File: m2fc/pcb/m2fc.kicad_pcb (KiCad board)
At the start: 4 copper layers, 100 x 70 mm, 347 parts, among them IC101 ADP3335, IC102 STM32F405VGT, IC103 ADP3335, IC201 AD8226, IC202 AD8656, IC203 AD8541, IC204 AD8226, IC205 AD8656, IC206 AD8541, IC207 AD8226, IC208 AD8656, IC209 AD8541, IC301 ADXL375, IC302 ADXL345, IC303 MS5611-01BA03, IC304 HMC5883L, IC305 L3G4200D, IC401 ADuM5201, IC402 ADuM1201, IC601 AD8495, IC602 AD8656, IC603 AD8495, IC604 AD8656, IC605 AD8495, IC606 AD8656, P101 CONN_2, P102 CONN_2, P103 CONN_2, P104 SWD, P201 CONN_4, P202 CONN_4, P203 CONN_4, P401 CONN_4, P402 CONN_2, P403 CONN_4, P501 CONN_2, P502 CONN_2, P503 CONN_2, P601 CONN_2, P602 CONN_2, P603 CONN_2, Q501 MOSFET_P, Q502 MOSFET_N, Q503 MOSFET_P, Q504 MOSFET_N, Q505 MOSFET_P, Q506 MOSFET_N, U106 MICROSD, U107 MOUNT, U108 MOUNT, U109 MOUNT, U110 MOUNT, U111 MOUNT, U112 MOUNT, X101 8M

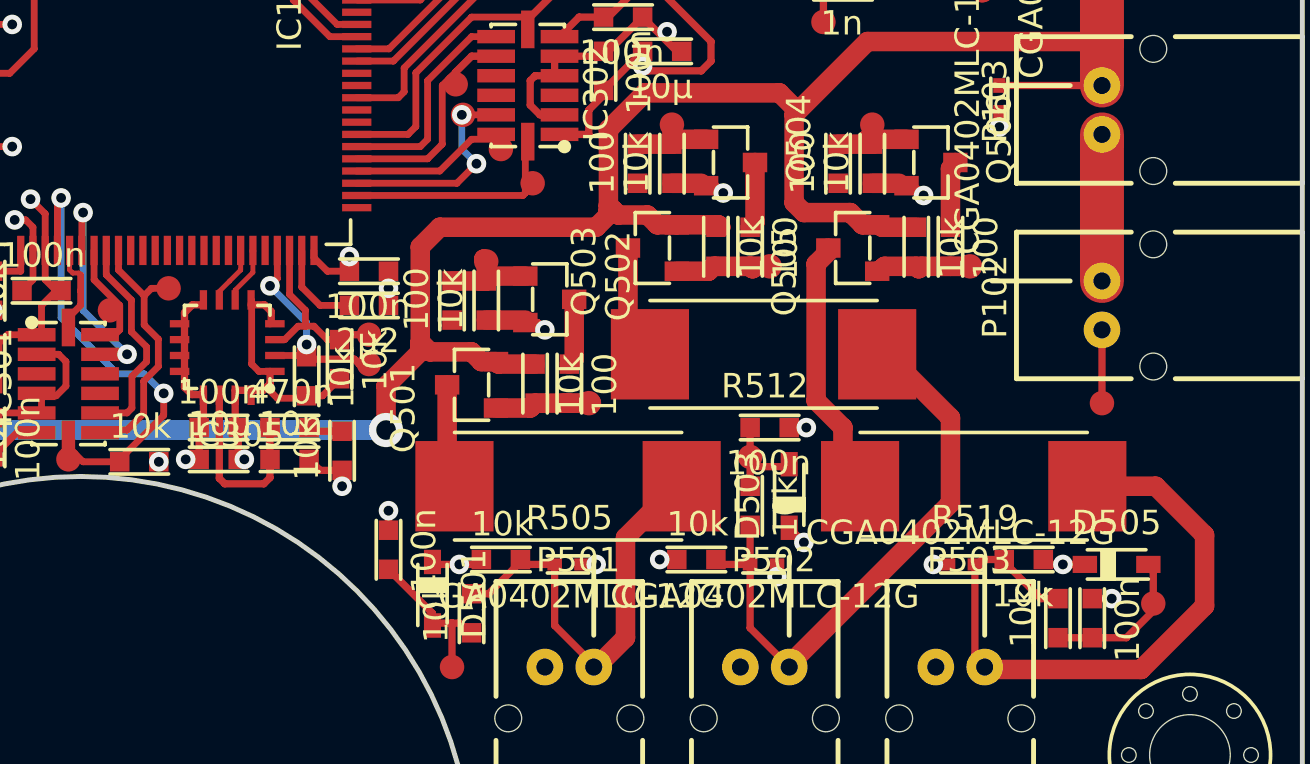
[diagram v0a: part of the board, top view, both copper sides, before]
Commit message: nc 0
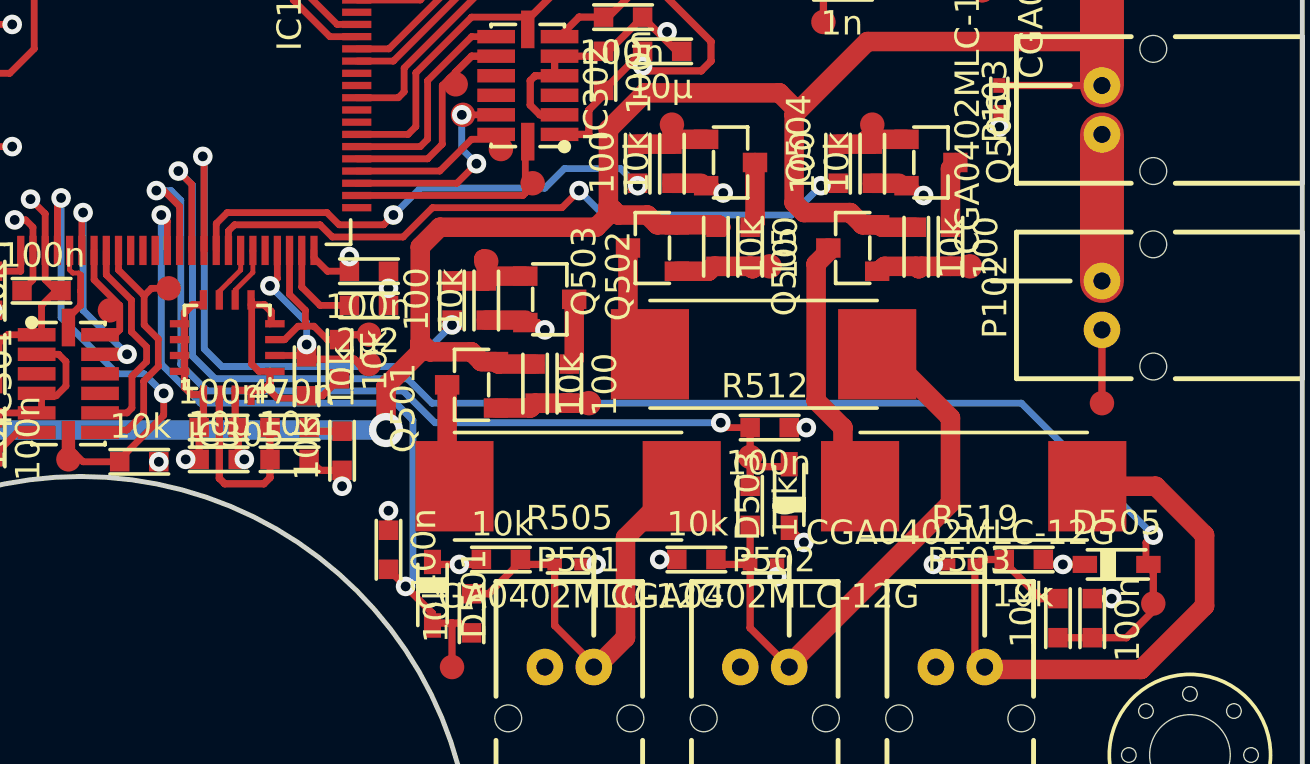
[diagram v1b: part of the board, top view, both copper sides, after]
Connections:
- IC102 pad 39: /Pyros/PYRO_1_F -> /Pyros/PYRO_2_C
- IC102 pad 40: /Pyros/PYRO_2_C -> /Pyros/PYRO_3_C
- IC102 pad 41: /Pyros/PYRO_2_F -> /Pyros/PYRO_1_F
- IC102 pad 42: /Pyros/PYRO_3_C -> /Pyros/PYRO_2_F
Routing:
- net /Pyros/PYRO_3_C: track 6.59 -> 61.6 mm, vias 0 -> 2
- net /Pyros/PYRO_2_C: track 4.51 -> 39.8 mm, vias 0 -> 2
- net /Pyros/PYRO_3_F: track 0.00 -> 27.8 mm, vias 0 -> 2
- net /Pyros/PYRO_1_C: track 6.65 -> 32.7 mm, vias 0 -> 2
- net /Pyros/PYRO_1_F: track 0.00 -> 23.1 mm, vias 0 -> 2
- net /Pyros/PYRO_2_F: track 0.00 -> 20.1 mm, vias 0 -> 2
